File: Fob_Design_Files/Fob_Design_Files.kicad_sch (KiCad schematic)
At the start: 30 parts, among them J2 Conn_02x04_Counter_Clockwise, U1 MAX16054AZT_T, U2 CC1101RGPR, U3 BU2032SM-JJ-GTR, U4 STM32C011F4Px, U5 TLV70028_SOT353, Y1 NX3225GA-26.000MHZ-EXS00A-CG0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

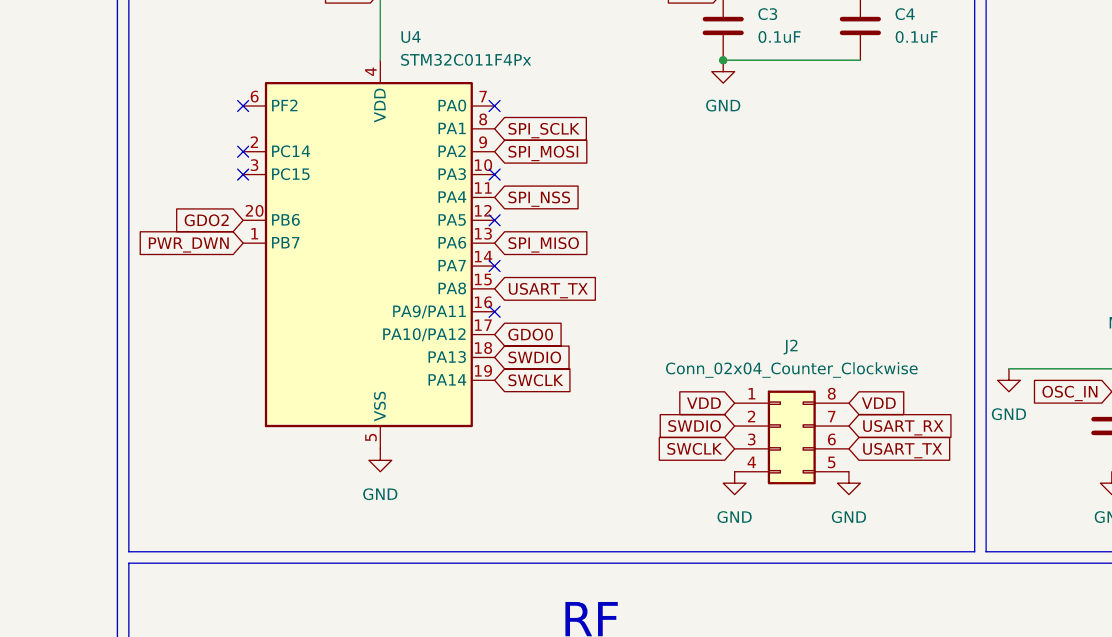
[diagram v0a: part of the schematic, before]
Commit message: Done with fob layout
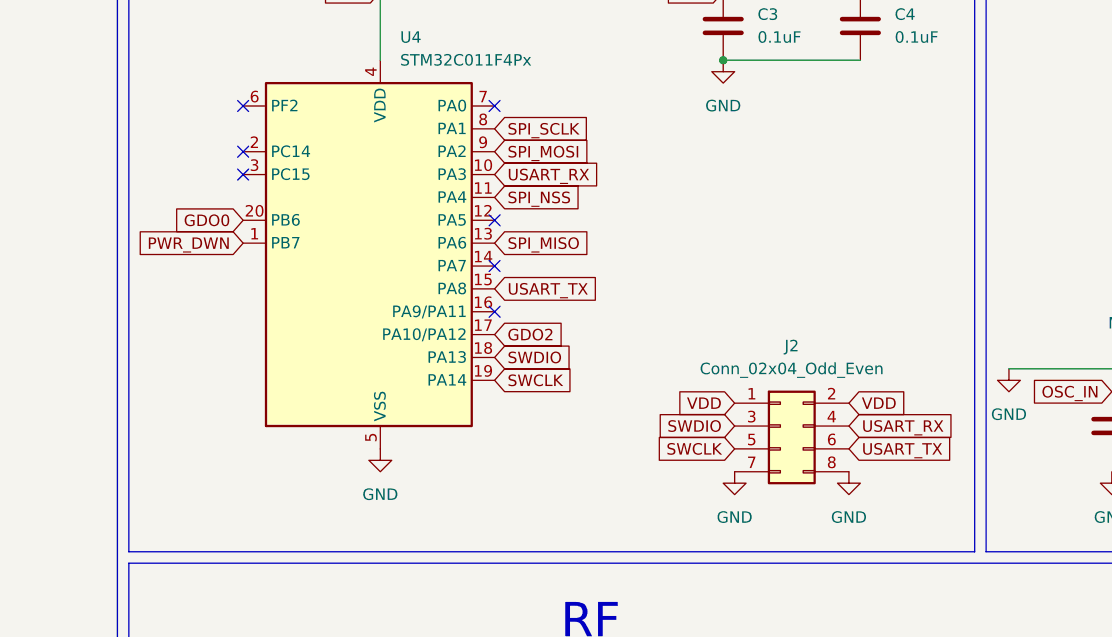
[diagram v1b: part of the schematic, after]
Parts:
- removed J2: Conn_02x04_Counter_Clockwise, Connector_PinSocket_2.54mm:PinSocket_2x04_P2.54mm_Vertical, symbol Connector_Generic:Conn_02x04_Counter_Clockwise
- added J2: Conn_02x04_Odd_Even, Connector_PinSocket_2.54mm:PinSocket_2x04_P2.54mm_Vertical, symbol Connector_Generic:Conn_02x04_Odd_Even
- C10, C11, C12, C13, C14, C15, C6, C7: footprint Capacitor_SMD:C_0402_1005Metric -> Capacitor_SMD:C_0603_1608Metric
- L1, L2, L3, L4: footprint Inductor_SMD:L_0402_1005Metric -> Inductor_SMD:L_0603_1608Metric
- R1, R2: footprint Resistor_SMD:R_0402_1005Metric -> Inductor_SMD:L_0603_1608Metric
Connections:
- net GDO0: now also U4.20 (PB6); no longer U4.17 (PA10/PA12)
- net GDO2: now also U4.17 (PA10/PA12); no longer U4.20 (PB6)
- net GND: now also J2.7 (Pin_7), J2.8 (Pin_8)
- net SWCLK: now also J2.5 (Pin_5)
- net SWDIO: now also J2.3 (Pin_3)
- net USART_RX: now also U4.10 (PA3), J2.4 (Pin_4)
- net USART_TX: now also J2.6 (Pin_6)
- net VDD: now also J2.1 (Pin_1), J2.2 (Pin_2)
- no-connect marks 10 -> 9
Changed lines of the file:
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@@
 	)
 	(no_connect
-		(at 199.39 57.15)
-	)
-	(no_connect
 		(at 199.39 49.53)
 	)
@@
 		)
 	)
-	(global_label "GDO2"
-		(shape input)
-		(at 171.45 62.23 180)
-		(fields_autoplaced yes)
-		(effects
-			(font
-				(size 1.27 1.27)
-			)
-			(justify right)
-		)
-		(property "Intersheetrefs" "${INTERSHEET_REFS}"
-			(at 163.3848 62.23 0)
-			(effects
-				(font
-					(size 1.27 1.27)
-				)
-				(justify right)
-				(hide yes)
-			)
-		)
-	)
 	(global_label "Button"
 		(shape input)
@@
 		)
 	)
+	(global_label "USART_RX"
+		(shape input)
+		(at 238.76 85.09 0)
+		(fields_autoplaced yes)
+		(effects
+			(font
+				(size 1.27 1.27)
+			)
+			(justify left)
+		)
+		(property "Intersheetrefs" "${INTERSHEET_REFS}"
+			(at 251.0585 85.09 0)
+			(effects
+				(font
+					(size 1.27 1.27)
+				)
+				(justify left)
+				(hide yes)
+			)
+		)
+	)
 	(global_label "SPI_NSS"
 		(shape input)
@@
 		)
 	)
+	(global_label "USART_RX"
+		(shape input)
+		(at 199.39 57.15 0)
+		(fields_autoplaced yes)
+		(effects
+			(font
+				(size 1.27 1.27)
+			)
+			(justify left)
+		)
+		(property "Intersheetrefs" "${INTERSHEET_REFS}"
+			(at 211.6885 57.15 0)
+			(effects
+				(font
+					(size 1.27 1.27)
+				)
+				(justify left)
+				(hide yes)
+			)
+		)
+	)
 	(global_label "PWR_DWN"
 		(shape input)
@@
 		)
 	)
-	(global_label "USART_RX"
+	(global_label "VDD"
 		(shape input)
-		(at 238.76 85.09 0)
+		(at 374.65 58.42 0)
 		(fields_autoplaced yes)
 		(effects
@@
 		)
 		(property "Intersheetrefs" "${INTERSHEET_REFS}"
-			(at 251.0585 85.09 0)
+			(at 381.2638 58.42 0)
 			(effects
 				(font
@@
 	(global_label "VDD"
 		(shape input)
-		(at 374.65 58.42 0)
+		(at 374.65 50.8 0)
 		(fields_autoplaced yes)
 		(effects
@@
 		)
 		(property "Intersheetrefs" "${INTERSHEET_REFS}"
-			(at 381.2638 58.42 0)
+			(at 381.2638 50.8 0)
 			(effects
 				(font
@@
 		)
 	)
-	(global_label "VDD"
+	(global_label "GDO0"
 		(shape input)
-		(at 374.65 50.8 0)
+		(at 171.45 62.23 180)
 		(fields_autoplaced yes)
 		(effects
@@
 				(size 1.27 1.27)
 			)
-			(justify left)
+			(justify right)
 		)
 		(property "Intersheetrefs" "${INTERSHEET_REFS}"
-			(at 381.2638 50.8 0)
+			(at 163.3848 62.23 0)
 			(effects
 				(font
 					(size 1.27 1.27)
 				)
-				(justify left)
+				(justify right)
 				(hide yes)
 			)
@@
 		)
 	)
+	(global_label "GDO2"
+		(shape input)
+		(at 199.39 74.93 0)
+		(fields_autoplaced yes)
+		(effects
+			(font
+				(size 1.27 1.27)
+			)
+			(justify left)
+		)
+		(property "Intersheetrefs" "${INTERSHEET_REFS}"
+			(at 207.4552 74.93 0)
+			(effects
+				(font
+					(size 1.27 1.27)
+				)
+				(justify left)
+				(hide yes)
+			)
+		)
+	)
 	(global_label "PWR_DWN"
 		(shape input)
@@
 		)
 	)
-	(global_label "GDO0"
-		(shape input)
-		(at 199.39 74.93 0)
-		(fields_autoplaced yes)
-		(effects
-			(font
-				(size 1.27 1.27)
-			)
-			(justify left)
-		)
-		(property "Intersheetrefs" "${INTERSHEET_REFS}"
-			(at 207.4552 74.93 0)
-			(effects
-				(font
-					(size 1.27 1.27)
-				)
-				(justify left)
-				(hide yes)
-			)
-		)
-	)
 	(global_label "SPI_MOSI"
 		(shape input)
@@
 	)
 	(symbol
-		(lib_id "Connector_Generic:Conn_02x04_Counter_Clockwise")
+		(lib_id "Connector_Generic:Conn_02x04_Odd_Even")
 		(at 231.14 85.09 0)
 		(unit 1)
@@
 			)
 		)
-		(property "Value" "Conn_02x04_Counter_Clockwise"
+		(property "Value" "Conn_02x04_Odd_Even"
 			(at 232.41 78.74 0)
 			(effects
@@
 			)
 		)
-		(property "Description" "Generic connector, double row, 02x04, counter clockwise pin numbering scheme (similar to DIP package numbering), script generated (kicad-library-utils/schlib/autogen/connector/)"
+		(property "Description" "Generic connector, double row, 02x04, odd/even pin numbering scheme (row 1 odd numbers, row 2 even numbers), script generated (kicad-library-utils/schlib/autogen/connector/)"
 			(at 231.14 85.09 0)
 			(effects
@@
 			)
 		)
-		(pin "3"
-		)
-		(pin "1"
+		(pin "5"
 		)
-		(pin "2"
+		(pin "3"
 		)
-		(pin "6"
+		(pin "7"
 		)
 		(pin "4"
 		)
-		(pin "5"
+		(pin "1"
 		)
-		(pin "7"
+		(pin "2"
 		)
 		(pin "8"
 		)
+		(pin "6"
+		)
 		(instances
 			(project ""
@@
 			)
 		)
-		(property "Footprint" "Inductor_SMD:L_0402_1005Metric"
+		(property "Footprint" "Inductor_SMD:L_0603_1608Metric"
 			(at 181.61 147.32 0)
 			(effects
@@
 			)
 		)
-		(property "Footprint" "Resistor_SMD:R_0402_1005Metric"
+		(property "Footprint" "Inductor_SMD:L_0603_1608Metric"
 			(at 39.878 105.41 90)
 			(effects
@@
 			)
 		)
-		(property "Footprint" "Resistor_SMD:R_0402_1005Metric"
+		(property "Footprint" "Inductor_SMD:L_0603_1608Metric"
 			(at 347.98 83.058 90)
 			(effects
@@
 			)
 		)
-		(property "Footprint" "Capacitor_SMD:C_0402_1005Metric"
+		(property "Footprint" "Capacitor_SMD:C_0603_1608Metric"
 			(at 179.3748 120.65 0)
 			(effects
@@
 	(symbol
 		(lib_id "power:GND")
+		(at 238.76 90.17 0)
+		(unit 1)
+		(exclude_from_sim no)
+		(in_bom yes)
+		(on_board yes)
+		(dnp no)
+		(property "Reference" "#PWR09"
+			(at 238.76 96.52 0)
+			(effects
+				(font
+					(size 1.27 1.27)
+				)
+				(hide yes)
+			)
+		)
+		(property "Value" "GND"
+			(at 238.76 95.25 0)
+			(effects
+				(font
+					(size 1.27 1.27)
+				)
+			)
+		)
+		(property "Footprint" ""
+			(at 238.76 90.17 0)
+			(effects
+				(font
+					(size 1.27 1.27)
+				)
+				(hide yes)
+			)
+		)
+		(property "Datasheet" ""
+			(at 238.76 90.17 0)
+			(effects
+				(font
+					(size 1.27 1.27)
+				)
+				(hide yes)
+			)
+		)
+		(property "Description" "Power symbol creates a global label with name \"GND\" , ground"
+			(at 238.76 90.17 0)
+			(effects
+				(font
+					(size 1.27 1.27)
+				)
+				(hide yes)
+			)
+		)
+		(pin "1"
+		)
+		(instances
+			(project "Fob_Design_Files"
+				(path "/ad2bc408-bf54-4f88-a5fb-85c0e9c3efbd"
+					(reference "#PWR09")
+					(unit 1)
+				)
+			)
+		)
+	)
+	(symbol
+		(lib_id "power:GND")
 		(at 231.14 143.51 0)
 		(unit 1)
@@
 			)
 		)
-		(property "Footprint" "Capacitor_SMD:C_0402_1005Metric"
+		(property "Footprint" "Capacitor_SMD:C_0603_1608Metric"
 			(at 230.1748 135.89 0)
 			(effects
@@
 			)
 		)
-		(property "Footprint" "Capacitor_SMD:C_0402_1005Metric"
+		(property "Footprint" "Capacitor_SMD:C_0603_1608Metric"
 			(at 268.9352 88.9 0)
 			(effects
@@
 			)
 		)
-		(property "Footprint" "Capacitor_SMD:C_0402_1005Metric"
+		(property "Footprint" "Capacitor_SMD:C_0603_1608Metric"
 			(at 310.8452 86.36 0)
 			(effects
@@
 			)
 		)
-		(property "Footprint" "Capacitor_SMD:C_0402_1005Metric"
+		(property "Footprint" "Capacitor_SMD:C_0603_1608Metric"
 			(at 190.5 144.4752 0)
 			(effects
@@
 			)
 		)
-		(property "Footprint" "Capacitor_SMD:C_0402_1005Metric"
+		(property "Footprint" "Capacitor_SMD:C_0603_1608Metric"
 			(at 248.92 134.9248 0)
 			(effects
@@
 			)
 		)
-		(property "Footprint" "Inductor_SMD:L_0402_1005Metric"
+		(property "Footprint" "Inductor_SMD:L_0603_1608Metric"
 			(at 205.74 135.89 0)
 			(effects
@@
 			)
 		)
-		(property "Footprint" "Inductor_SMD:L_0402_1005Metric"
+		(property "Footprint" "Inductor_SMD:L_0603_1608Metric"
 			(at 194.31 128.27 0)
 			(effects
@@
 			)
 		)
-		(property "Footprint" "Capacitor_SMD:C_0402_1005Metric"
+		(property "Footprint" "Capacitor_SMD:C_0603_1608Metric"
 			(at 180.6448 151.13 0)
 			(effects
@@
 			)
 		)
-		(property "Footprint" "Capacitor_SMD:C_0402_1005Metric"
+		(property "Footprint" "Capacitor_SMD:C_0603_1608Metric"
 			(at 212.3948 135.89 0)
 			(effects
@@
 	(symbol
 		(lib_id "power:GND")
-		(at 238.76 90.17 0)
-		(unit 1)
-		(exclude_from_sim no)
-		(in_bom yes)
-		(on_board yes)
-		(dnp no)
-		(fields_autoplaced yes)
-		(property "Reference" "#PWR029"
-			(at 238.76 96.52 0)
-			(effects
-				(font
-					(size 1.27 1.27)
-				)
-				(hide yes)
-			)
-		)
-		(property "Value" "GND"
-			(at 238.76 95.25 0)
-			(effects
-				(font
-					(size 1.27 1.27)
-				)
-			)
-		)
-		(property "Footprint" ""
-			(at 238.76 90.17 0)
-			(effects
-				(font
-					(size 1.27 1.27)
-				)
-				(hide yes)
-			)
-		)
-		(property "Datasheet" ""
-			(at 238.76 90.17 0)
-			(effects
-				(font
-					(size 1.27 1.27)
-				)
-				(hide yes)
-			)
-		)
-		(property "Description" "Power symbol creates a global label with name \"GND\" , ground"
-			(at 238.76 90.17 0)
-			(effects
-				(font
-					(size 1.27 1.27)
-				)
-				(hide yes)
-			)
-		)
-		(pin "1"
-		)
-		(instances
-			(project "Fob_Design_Files"
-				(path "/ad2bc408-bf54-4f88-a5fb-85c0e9c3efbd"
-					(reference "#PWR029")
-					(unit 1)
-				)
-			)
-		)
-	)
-	(symbol
-		(lib_id "power:GND")
 		(at 256.54 78.74 0)
 		(unit 1)
@@
 			)
 		)
-		(property "Footprint" "Inductor_SMD:L_0402_1005Metric"
+		(property "Footprint" "Inductor_SMD:L_0603_1608Metric"
 			(at 222.25 135.89 0)
 			(effects

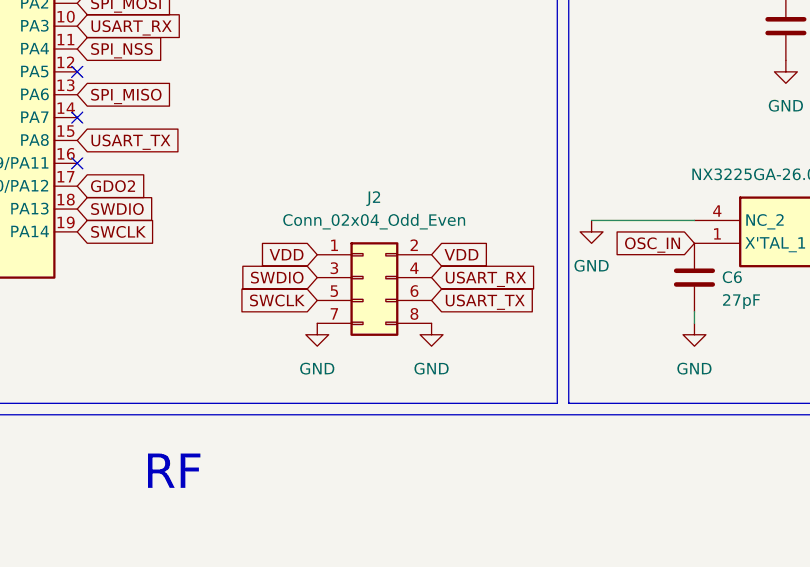
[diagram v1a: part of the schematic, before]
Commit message: Minor changes
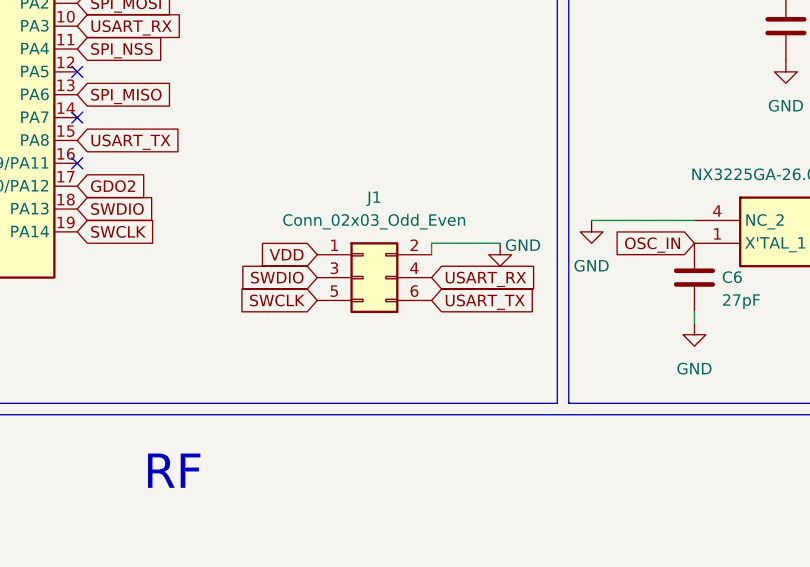
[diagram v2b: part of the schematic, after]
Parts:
- removed J2: Conn_02x04_Odd_Even, Connector_PinSocket_2.54mm:PinSocket_2x04_P2.54mm_Vertical, symbol Connector_Generic:Conn_02x04_Odd_Even
- added J1: Conn_02x03_Odd_Even, Connector_PinSocket_2.54mm:PinSocket_2x03_P2.54mm_Vertical, symbol Connector_Generic:Conn_02x03_Odd_Even
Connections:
- net GND: now also J1.2 (Pin_2)
- net SWCLK: now also J1.5 (Pin_5)
- net SWDIO: now also J1.3 (Pin_3)
- net USART_RX: now also J1.4 (Pin_4)
- net USART_TX: now also J1.6 (Pin_6)
- net VDD: now also J1.1 (Pin_1)
